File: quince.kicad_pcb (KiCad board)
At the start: 2 copper layers, 70.7 x 53.3 mm, 26 parts, among them J1 NEIGHBOR1, J2 NEIGHBOR2, J7 BONUS_ROW, P9 BASEBAND, U1 TLV3502

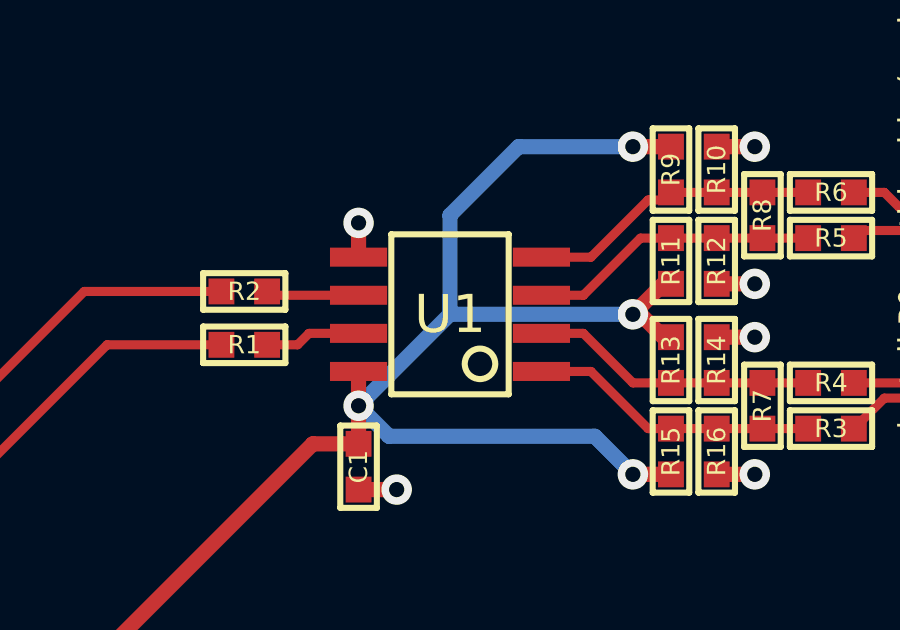
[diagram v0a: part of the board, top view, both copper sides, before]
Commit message: assign footprints
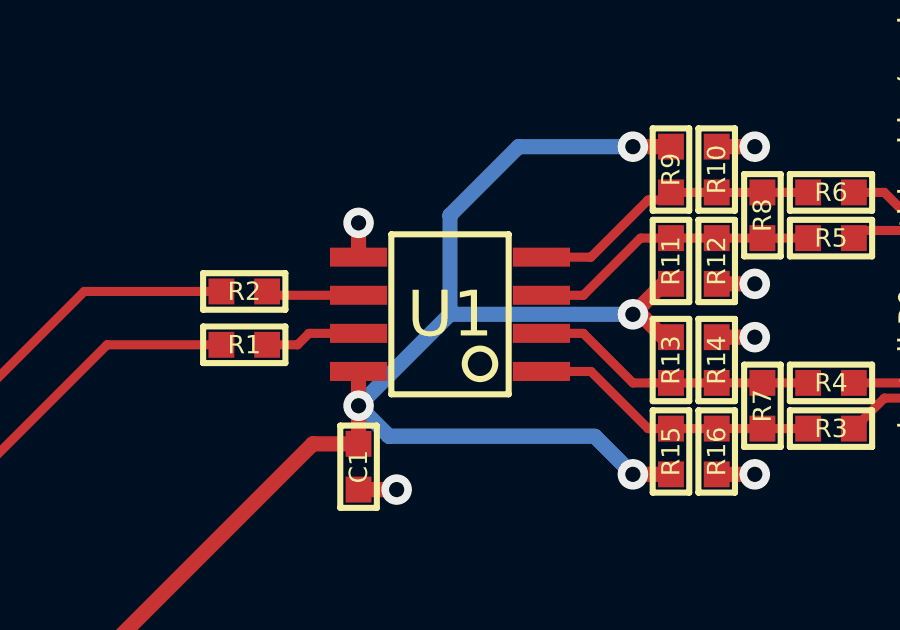
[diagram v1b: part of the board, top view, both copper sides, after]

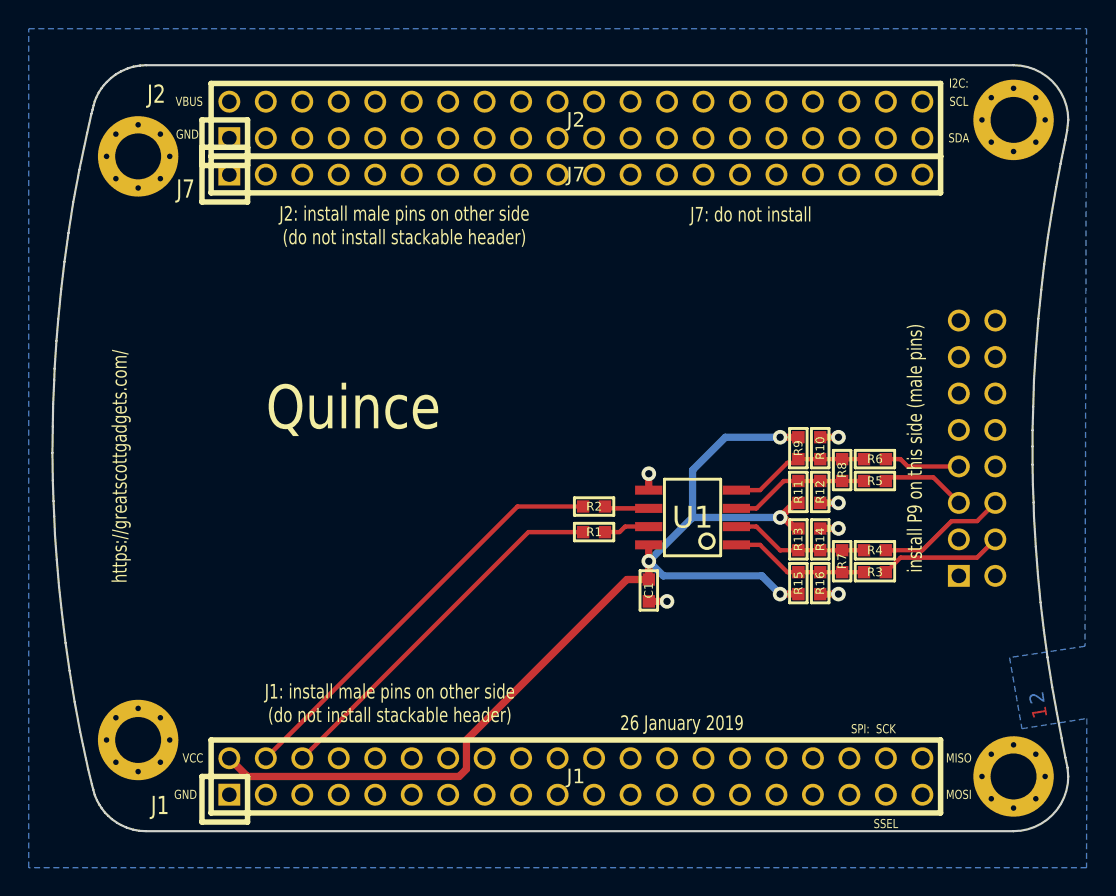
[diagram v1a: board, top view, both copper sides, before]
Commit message: complete layout
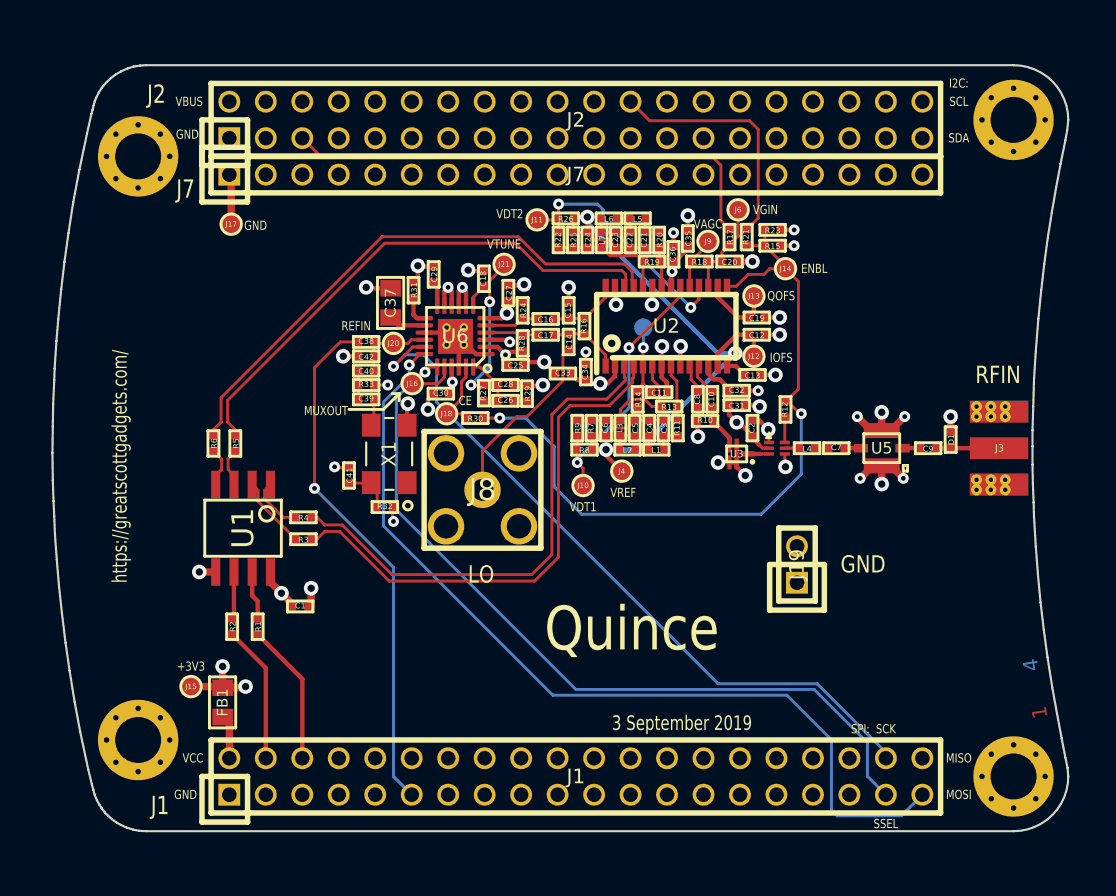
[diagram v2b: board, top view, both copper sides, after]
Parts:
- removed P9: BASEBAND, gsg-modules:HEADER-2x8
- added C10: 100pF, gsg-modules:0402, F.Cu at (155.6, 91.8)
- added C11: 100nF, gsg-modules:0402, F.Cu at (151.8, 91.3)
- added C12: 100nF, gsg-modules:0402, F.Cu at (158.7, 87.3)
- added C13: 100nF, gsg-modules:0402, F.Cu at (158.3, 90.2)
- added C14: 100pF, gsg-modules:0402, F.Cu at (145.6, 87.8)
- added C15: 100pF, gsg-modules:0402, F.Cu at (145.6, 85.7)
- added C16: 100pF, gsg-modules:0402, F.Cu at (143.9, 86.2)
- added C17: 100pF, gsg-modules:0402, F.Cu at (143.9, 87.3)
- added C18: 270pF, gsg-modules:0402, F.Cu at (139.7, 83.5)
- added C19: 100nF, gsg-modules:0402, F.Cu at (158.7, 86.2)
- added C2: 1nF, gsg-modules:0402, F.Cu at (158.3, 93.8)
- added C20: 100nF, gsg-modules:0402, F.Cu at (156.8, 82.2)
- added C21: 18pF, gsg-modules:0402, F.Cu at (150.8, 80.8)
- added C22: 68pF, gsg-modules:0402, F.Cu at (149.8, 80.8)
- added C23: 68pF, gsg-modules:0402, F.Cu at (148.8, 80.8)
- added C24: 18pF, gsg-modules:0402, F.Cu at (146.8, 80.8)
- added C25: 100nF, gsg-modules:0402, F.Cu at (141.8, 89.5)
- added C26: 8.2nF, gsg-modules:0402, F.Cu at (141.2, 92.0)
- added C27: 100nF, gsg-modules:0402, F.Cu at (141.3, 84.5)
- added C28: 560pF, gsg-modules:0402, F.Cu at (141.2, 90.8)
- added C29: 10nF, gsg-modules:0402, F.Cu at (136.2, 83.2)
- added C3: 18pF, gsg-modules:0402, F.Cu at (152.2, 93.8)
- added C30: 100nF, gsg-modules:0402, F.Cu at (136.7, 91.5)
- added C31: 100nF, gsg-modules:0402, F.Cu at (157.2, 92.2)
- added C32: 100pF, gsg-modules:0402, F.Cu at (157.2, 91.2)
- added C33: 100nF, gsg-modules:0402, F.Cu at (145.2, 90.0)
- added C34: 100pF, gsg-modules:0402, F.Cu at (146.8, 90.0)
- added C35: 100nF, gsg-modules:0402, F.Cu at (153.8, 80.7)
- added C36: 100pF, gsg-modules:0402, F.Cu at (152.8, 81.8)
- added C37: 10uF, gsg-modules:0805, F.Cu at (133.2, 85.1)
- added C38: C, gsg-modules:0402, F.Cu at (131.4, 87.8)
- added C39: 1nF, gsg-modules:0402, F.Cu at (131.4, 91.8)
- added C4: 68pF, gsg-modules:0402, F.Cu at (151.2, 93.8)
- added C40: 1nF, gsg-modules:0402, F.Cu at (131.4, 89.8)
- added C41: 100nF, gsg-modules:0402, F.Cu at (130.2, 97.2)
- added C42: C, gsg-modules:0402, F.Cu at (131.4, 88.8)
- added C5: 68pF, gsg-modules:0402, F.Cu at (150.2, 93.8)
- added C6: 18pF, gsg-modules:0402, F.Cu at (148.2, 93.8)
- added C7: 1nF, gsg-modules:0402, F.Cu at (164.2, 95.2)
- added C8: 100pF, gsg-modules:0402, F.Cu at (154.6, 91.8)
- added C9: 100pF, gsg-modules:0402, F.Cu at (170.6, 95.2)
- added D1: D_TVS, gsg-modules:0402, F.Cu at (172.2, 94.7)
- added FB1: Ferrite_Bead, gsg-modules:0805, F.Cu at (121.5, 113.0)
- added J10: Conn_01x01, gsg-modules:TESTPOINT-50MIL, F.Cu at (146.6, 97.8)
- added J11: Conn_01x01, gsg-modules:TESTPOINT-50MIL, F.Cu at (143.3, 79.3)
- added J12: Conn_01x01, gsg-modules:TESTPOINT-50MIL, F.Cu at (158.4, 88.8)
- added J13: Conn_01x01, gsg-modules:TESTPOINT-50MIL, F.Cu at (158.4, 84.7)
- added J14: Conn_01x01, gsg-modules:TESTPOINT-50MIL, F.Cu at (160.7, 82.8)
- added J15: Conn_01x01, gsg-modules:TESTPOINT-50MIL, F.Cu at (119.2, 111.8)
- added J16: Conn_01x01, gsg-modules:TESTPOINT-50MIL, F.Cu at (134.7, 90.8)
- added J17: Conn_01x01, gsg-modules:TESTPOINT-50MIL, F.Cu at (122.0, 79.7)
- added J18: Conn_01x01, gsg-modules:TESTPOINT-50MIL, F.Cu at (137.1, 92.8)
- added J19: GND, gsg-modules:HEADER-1x2, F.Cu at (161.4, 103.3)
- added J20: Conn_01x01, gsg-modules:TESTPOINT-50MIL, F.Cu at (133.3, 88.0)
- added J21: Conn_01x01, gsg-modules:TESTPOINT-50MIL, F.Cu at (141.1, 82.5)
- added J3: RFIN, gsg-modules:SMA-EDGE, F.Cu at (177.6, 95.2)
- added J4: Conn_01x01, gsg-modules:TESTPOINT-50MIL, F.Cu at (149.2, 96.8)
- added J5: Conn_01x01, gsg-modules:TESTPOINT-50MIL, B.Cu at (150.8, 86.8)
- added J6: Conn_01x01, gsg-modules:TESTPOINT-50MIL, F.Cu at (157.3, 78.7)
- added J8: LO, gsg-modules:SMA-VERTICAL, F.Cu at (139.6, 98.2)
- added J9: Conn_01x01, gsg-modules:TESTPOINT-50MIL, F.Cu at (155.2, 80.8)
- added L1: 470nH, gsg-modules:0402, F.Cu at (151.7, 95.3)
- added L2: 680nH, gsg-modules:0402, F.Cu at (149.7, 95.3)
- added L3: 470nH, gsg-modules:0402, F.Cu at (149.2, 93.8)
- added L4: 3.6nH, gsg-modules:0402, F.Cu at (162.2, 95.2)
- added L5: 470nH, gsg-modules:0402, F.Cu at (150.3, 79.2)
- added L6: 680nH, gsg-modules:0402, F.Cu at (148.3, 79.2)
- added L7: 470nH, gsg-modules:0402, F.Cu at (147.8, 80.8)
- added R17: 0, gsg-modules:0402, F.Cu at (156.8, 80.5)
- added R18: 0, gsg-modules:0402, F.Cu at (154.7, 82.2)
- added R19: 0, gsg-modules:0402, F.Cu at (151.3, 82.2)
- added R20: 100, gsg-modules:0402, F.Cu at (151.8, 80.8)
- added R21: 0, gsg-modules:0402, F.Cu at (157.9, 80.5)
- added R22: 2k2, gsg-modules:0402, F.Cu at (144.8, 80.8)
- added R23: 10k, gsg-modules:0402, F.Cu at (159.8, 80.0)
- added R24: 51, gsg-modules:0402, F.Cu at (142.3, 85.7)
- added R25: 100, gsg-modules:0402, F.Cu at (145.8, 80.8)
- added R26: 3k3, gsg-modules:0402, F.Cu at (145.3, 79.2)
- added R27: 3k, gsg-modules:0402, F.Cu at (139.7, 91.4)
- added R28: 51, gsg-modules:0402, F.Cu at (142.3, 88.0)
- added R29: 1.5k, gsg-modules:0402, F.Cu at (142.7, 91.5)
- added R30: 0, gsg-modules:0402, F.Cu at (139.1, 93.2)
- added R31: 3k3, gsg-modules:0402, F.Cu at (134.8, 84.2)
- added R32: 0, gsg-modules:0402, F.Cu at (132.8, 99.3)
- added R33: 51, gsg-modules:0402, F.Cu at (131.4, 90.8)
- added U2: AD8347, gsg-modules:TSSOP28, F.Cu at (152.3, 86.8)
- added U3: SAW FILTER, gsg-modules:B9413, F.Cu at (157.2, 95.7)
- added U4: LNA, gsg-modules:BGA7H1N6, F.Cu at (160.1, 95.2)
- added U5: BAND PASS FILTER, gsg-modules:2450BP39D100C, F.Cu at (167.3, 95.2)
- added U6: ADF4360, gsg-modules:QFN24-4, F.Cu at (137.7, 87.5)
- added X1: TCXO, gsg-modules:XTAL5.0x3.2mm, F.Cu at (133.1, 95.7)
- C1: value C -> 100nF; footprint gsg-modules:0603 -> gsg-modules:0402
- R1, R2, R3, R4, R5, R6: footprint gsg-modules:0603 -> gsg-modules:0402
- R10, R16: value R -> 200; footprint gsg-modules:0603 -> gsg-modules:0402
- R11, R7: value R -> 100; footprint gsg-modules:0603 -> gsg-modules:0402
- R12, R13, R14: value R -> 0; footprint gsg-modules:0603 -> gsg-modules:0402
- R15: value R -> 10k; footprint gsg-modules:0603 -> gsg-modules:0402
- R8: value R -> 3k3; footprint gsg-modules:0603 -> gsg-modules:0402
- R9: value R -> 2k2; footprint gsg-modules:0603 -> gsg-modules:0402
- moved R6 46.1 mm to (120.8, 94.9), turned to 90 degrees
- moved R5 44.6 mm to (122.3, 94.9), turned to 90 degrees
- moved R3 39.9 mm to (127.1, 101.6)
- moved R4 39.9 mm to (127.1, 100.1)
- moved U1 31.3 mm to (122.9, 100.8), turned to 270 degrees
- moved R2 26.6 mm to (122.1, 107.7), turned to 90 degrees
- moved R1 24.3 mm to (123.9, 107.7), turned to 90 degrees
- moved C1 24.3 mm to (126.9, 106.3), turned to 180 degrees
- moved R16 24.3 mm to (146.7, 86.8)
- moved R15 23.6 mm to (159.8, 81.2), turned to 0 degrees
- moved R7 19.8 mm to (147.2, 93.8), turned to 270 degrees
- moved R8 18.0 mm to (146.7, 95.3), turned to 0 degrees
- moved R14 16.0 mm to (150.3, 91.8)
- moved R9 15.5 mm to (146.2, 93.8), turned to 90 degrees
- moved R13 12.9 mm to (152.6, 92.3), turned to 0 degrees
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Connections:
- C1 pad 2: VCC -> +3V3
- J1 pad 11: (no net) -> /CLK0
- J1 pad 37: (no net) -> /P1_20
- J1 pad 38: (no net) -> /P1_19
- J1 pad 39: (no net) -> /P1_4
- J2 pad 24: (no net) -> /P3_1
- J2 pad 5: (no net) -> /ADC0_0
- R10 pad 1: /-IN_B -> Net-(C10-Pad2)
- R11 pad 1: VCC -> /IMXO
- R11 pad 2: /+IN_B -> Net-(C3-Pad1)
- R12 pad 1: /+IN_B -> /ENBL
- R12 pad 2: GND -> Net-(R12-Pad2)
- R13 pad 1: VCC -> /IAIN
- R13 pad 2: /-IN_A -> /IMXO
- R14 pad 1: /-IN_A -> /VREF
- R14 pad 2: GND -> /VCMO
- R15 pad 1: VCC -> /ENBL
- R15 pad 2: /+IN_A -> +3V3
- R16 pad 1: /+IN_A -> /LOI_P
- R16 pad 2: GND -> /LOI_N
- R3 pad 1: /+IN_A -> /IN_A+
- R3 pad 2: /RXBBQ- -> /IOP_P
- R4 pad 1: /-IN_A -> /IN_A-
- R4 pad 2: /RXBBQ+ -> /IOP_N
- R5 pad 1: /+IN_B -> /IN_B+
- R5 pad 2: /RXBBI- -> /QOP_N
- R6 pad 1: /-IN_B -> /IN_B-
- R6 pad 2: /RXBBI+ -> /QOP_P
- R7 pad 1: /+IN_A -> /IAIN
- R7 pad 2: /-IN_A -> /VREF
- R8 pad 1: /+IN_B -> /VDT1
- R8 pad 2: /-IN_B -> /VREF
- R9 pad 1: VCC -> /VDT1
- R9 pad 2: /-IN_B -> /IAIN
- U1 pad 1: /+IN_A -> /IN_A-
- U1 pad 2: /-IN_A -> /IN_A+
- U1 pad 3: /+IN_B -> /IN_B+
- U1 pad 4: /-IN_B -> /IN_B-
- U1 pad 8: VCC -> +3V3
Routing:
- net VCC: track 75.7 -> 3.07 mm, vias 4 -> 0
- net GND: track 7.49 -> 74.5 mm, vias 6 -> 42
- net /P1_4: track 0.00 -> 62.7 mm, vias 0 -> 1
- net /P1_20: track 0.00 -> 55.2 mm, vias 0 -> 1
- net /ENBL: track 0.00 -> 52.6 mm, vias 0 -> 2
- net /P1_19: track 0.00 -> 50.6 mm, vias 0 -> 1
- net /VREF: track 0.00 -> 47.7 mm, vias 0 -> 3
- net /QOP_P: track 0.00 -> 38.2 mm
- net +3V3: track 0.00 -> 37.1 mm, vias 0 -> 12
- net /QOP_N: track 0.00 -> 36.7 mm
- net /IOP_P: track 0.00 -> 36.7 mm
- net /CLK0: track 0.00 -> 36.3 mm, vias 0 -> 1
- net /IOP_N: track 0.00 -> 35.9 mm
- net /ADC0_0: track 0.00 -> 34.6 mm
- net /P0_0: track 29.4 -> 9.60 mm
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- added copper zone on In2.Cu, net +3V3
- added copper zone on In1.Cu, net GND
- removed copper zone on B.Cu, net GND
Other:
- copper layers 2 -> 4
- net class Default: clearance 0.1524 -> 0.127
- rule trace_clearance: 0.1524 -> 0.127
- board text added: "+3V3"
- board text added: "3"
- board text added: "3 September 2019"
- board text added: "4"
- board text added: "CE"
- board text added: "ENBL"
- board text added: "IOFS"
- board text added: "LO"
- board text added: "MUXOUT"
- board text added: "QOFS"
- board text added: "REFIN"
- board text added: "VAGC"
- board text added: "VCMO"
- board text added: "VDT1"
- board text added: "VDT2"
- board text added: "VGIN"
- board text added: "VREF"
- board text added: "VTUNE"
- board text removed: "26 January 2019"
- board text removed: "J1: install male pins on other side (do not install stackable header)"
- board text removed: "J2: install male pins on other side (do not install stackable header)"
- board text removed: "J7: do not install"
- board text removed: "install P9 on other side"
- board text removed: "install P9 on this side (male pins)"
